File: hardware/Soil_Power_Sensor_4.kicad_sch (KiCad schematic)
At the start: 15 parts, among them J6 UART, SW1 EN, SW2 BOOT, U9 ESP32-C3-WROOM-02-N4

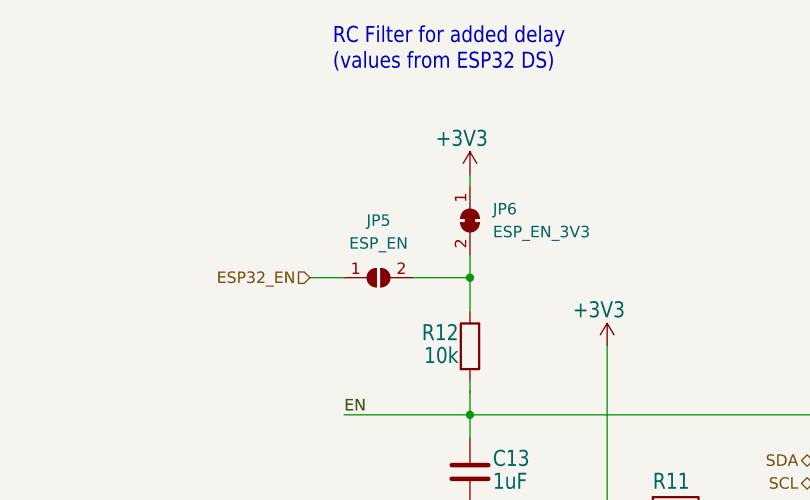
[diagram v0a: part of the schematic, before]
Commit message: Updated board layout
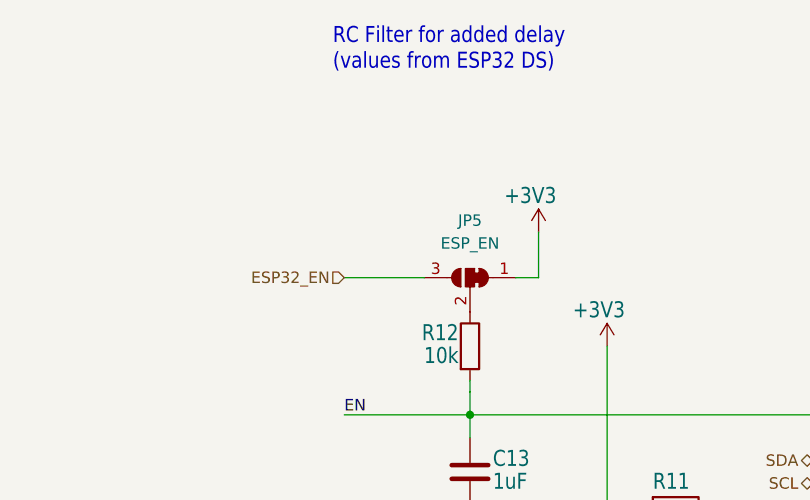
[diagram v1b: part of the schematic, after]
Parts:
- removed JP5: ESP_EN, symbol Jumper:SolderJumper_2_Open
- removed JP6: ESP_EN_3V3, symbol Jumper:SolderJumper_2_Bridged
- added JP5: ESP_EN, Jumper:SolderJumper-3_P1.3mm_Open_Pad1.0x1.5mm, symbol Jumper:SolderJumper_3_Bridged12
- JP4: footprint (none) -> Jumper:SolderJumper-2_P1.3mm_Open_Pad1.0x1.5mm
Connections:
- net +3V3: now also JP5.1 (A)
- net ESP32_EN: now also JP5.3 (B)
- net at R12.1: now also JP5.2 (C)
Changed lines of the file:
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@@
   (junction (at 187.96 106.68) (diameter 0) (color 0 0 0 0)
   )
-  (junction (at 106.68 63.5) (diameter 0) (color 0 0 0 0)
-  )
   (junction (at 210.82 68.58) (diameter 0) (color 0 0 0 0)
   )
   (junction (at 106.68 78.74) (diameter 0) (color 0 0 0 0)
   )
-  (wire (pts (xy 106.68 63.5) (xy 106.68 67.31))
-    (stroke (width 0) (type default))
-  )
   (wire (pts (xy 121.92 88.9) (xy 121.92 71.12))
     (stroke (width 0.1524) (type solid))
   )
-  (wire (pts (xy 106.68 52.07) (xy 106.68 53.34))
+  (wire (pts (xy 114.3 58.42) (xy 114.3 63.5))
     (stroke (width 0) (type default))
   )
@@
     (stroke (width 0) (type default))
   )
-  (wire (pts (xy 100.33 63.5) (xy 106.68 63.5))
-    (stroke (width 0.1524) (type solid))
-  )
   (wire (pts (xy 64.77 137.16) (xy 72.39 137.16))
     (stroke (width 0) (type default))
   )
-  (wire (pts (xy 88.9 63.5) (xy 92.71 63.5))
-    (stroke (width 0) (type default))
-  )
   (wire (pts (xy 220.98 68.58) (xy 210.82 68.58))
     (stroke (width 0.1524) (type solid))
@@
     (stroke (width 0) (type default))
   )
+  (wire (pts (xy 92.71 63.5) (xy 101.6 63.5))
+    (stroke (width 0) (type default))
+  )
   (wire (pts (xy 106.68 76.2) (xy 106.68 78.74))
     (stroke (width 0.1524) (type solid))
@@
     (stroke (width 0.1524) (type solid))
   )
+  (wire (pts (xy 114.3 63.5) (xy 111.76 63.5))
+    (stroke (width 0) (type default))
+  )
   (wire (pts (xy 210.82 76.2) (xy 210.82 68.58))
     (stroke (width 0.1524) (type solid))
@@
   )
   (wire (pts (xy 48.26 130.81) (xy 55.88 130.81))
-    (stroke (width 0) (type default))
-  )
-  (wire (pts (xy 106.68 60.96) (xy 106.68 63.5))
     (stroke (width 0) (type default))
   )
@@
     (effects (font (size 1.27 1.27)) (justify right))
   )
-  (hierarchical_label "ESP32_EN" (shape input) (at 88.9 63.5 180) (fields_autoplaced)
+  (hierarchical_label "ESP32_EN" (shape input) (at 92.71 63.5 180) (fields_autoplaced)
     (effects (font (size 1.27 1.27)) (justify right))
   )
@@
         (path "/5300ec4d-4648-40a1-8d89-4fa6b3bf32a3/1383843a-880b-4efd-8c7f-ecdf3639f794"
           (reference "C16") (unit 1)
-        )
-      )
-    )
-  )
-  (symbol (lib_id "Jumper:SolderJumper_2_Bridged") (at 106.68 57.15 270) (unit 1)
-    (in_bom yes) (on_board yes) (dnp no) (fields_autoplaced)
-    (property "Reference" "JP6" (at 109.22 55.88 90)
-      (effects (font (size 1.27 1.27)) (justify left))
-    )
-    (property "Value" "ESP_EN_3V3" (at 109.22 58.42 90)
-      (effects (font (size 1.27 1.27)) (justify left))
-    )
-    (property "Footprint" "" (at 106.68 57.15 0)
-      (effects (font (size 1.27 1.27)) hide)
-    )
-    (property "Datasheet" "~" (at 106.68 57.15 0)
-      (effects (font (size 1.27 1.27)) hide)
-    )
-    (pin "1")
-    (pin "2")
-    (instances
-      (project "Soil Power Sensor"
-        (path "/5300ec4d-4648-40a1-8d89-4fa6b3bf32a3/1383843a-880b-4efd-8c7f-ecdf3639f794"
-          (reference "JP6") (unit 1)
         )
       )
@@
     )
   )
-  (symbol (lib_id "Jumper:SolderJumper_2_Open") (at 96.52 63.5 0) (unit 1)
-    (in_bom yes) (on_board yes) (dnp no) (fields_autoplaced)
-    (property "Reference" "JP5" (at 96.52 57.15 0)
-      (effects (font (size 1.27 1.27)))
-    )
-    (property "Value" "ESP_EN" (at 96.52 59.69 0)
-      (effects (font (size 1.27 1.27)))
-    )
-    (property "Footprint" "" (at 96.52 63.5 0)
-      (effects (font (size 1.27 1.27)) hide)
-    )
-    (property "Datasheet" "~" (at 96.52 63.5 0)
-      (effects (font (size 1.27 1.27)) hide)
-    )
-    (pin "2")
-    (pin "1")
-    (instances
-      (project "Soil Power Sensor"
-        (path "/5300ec4d-4648-40a1-8d89-4fa6b3bf32a3/1383843a-880b-4efd-8c7f-ecdf3639f794"
-          (reference "JP5") (unit 1)
-        )
-      )
-    )
-  )
   (symbol (lib_id "power:+3V3") (at 121.92 71.12 0) (unit 1)
     (in_bom yes) (on_board yes) (dnp no)
@@
       (effects (font (size 1.27 1.27)))
     )
-    (property "Footprint" "" (at 81.28 130.81 0)
+    (property "Footprint" "Jumper:SolderJumper-2_P1.3mm_Open_Pad1.0x1.5mm" (at 81.28 130.81 0)
       (effects (font (size 1.27 1.27)) hide)
     )
@@
     )
   )
-  (symbol (lib_id "power:+3V3") (at 106.68 52.07 0) (unit 1)
-    (in_bom yes) (on_board yes) (dnp no)
-    (property "Reference" "#+3V09" (at 106.68 52.07 0)
-      (effects (font (size 1.27 1.27)) hide)
-    )
-    (property "Value" "+3V3" (at 102.87 46.99 0)
-      (effects (font (size 1.778 1.5113)) (justify left top))
-    )
-    (property "Footprint" "" (at 106.68 52.07 0)
-      (effects (font (size 1.27 1.27)) hide)
-    )
-    (property "Datasheet" "" (at 106.68 52.07 0)
+  (symbol (lib_id "power:+3V3") (at 114.3 58.42 0) (unit 1)
+    (in_bom yes) (on_board yes) (dnp no)
+    (property "Reference" "#+3V09" (at 114.3 58.42 0)
+      (effects (font (size 1.27 1.27)) hide)
+    )
+    (property "Value" "+3V3" (at 110.49 53.34 0)
+      (effects (font (size 1.778 1.5113)) (justify left top))
+    )
+    (property "Footprint" "" (at 114.3 58.42 0)
+      (effects (font (size 1.27 1.27)) hide)
+    )
+    (property "Datasheet" "" (at 114.3 58.42 0)
       (effects (font (size 1.27 1.27)) hide)
     )
@@
         )
       )
+    )
+  )
+  (symbol (lib_id "Jumper:SolderJumper_3_Bridged12") (at 106.68 63.5 0) (mirror y) (unit 1)
+    (in_bom yes) (on_board yes) (dnp no)
+    (property "Reference" "JP5" (at 106.68 57.15 0)
+      (effects (font (size 1.27 1.27)))
+    )
+    (property "Value" "ESP_EN" (at 106.68 59.69 0)
+      (effects (font (size 1.27 1.27)))
+    )
+    (property "Footprint" "Jumper:SolderJumper-3_P1.3mm_Open_Pad1.0x1.5mm" (at 106.68 63.5 0)
+      (effects (font (size 1.27 1.27)) hide)
+    )
+    (property "Datasheet" "~" (at 106.68 63.5 0)
+      (effects (font (size 1.27 1.27)) hide)
+    )
+    (pin "2")
+    (pin "3")
+    (pin "1")
+    (instances
+      (project "Soil Power Sensor"
+        (path "/5300ec4d-4648-40a1-8d89-4fa6b3bf32a3/1383843a-880b-4efd-8c7f-ecdf3639f794"
+          (reference "JP5") (unit 1)
+        )
+      )
